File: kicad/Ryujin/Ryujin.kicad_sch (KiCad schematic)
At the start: 17 parts, among them J3 BAT, J4 SDI12, Q1 IRLML6244, U1 TXS0101DBV, U2 R-78E5.0-0.5, U3 W25Q32JVSS

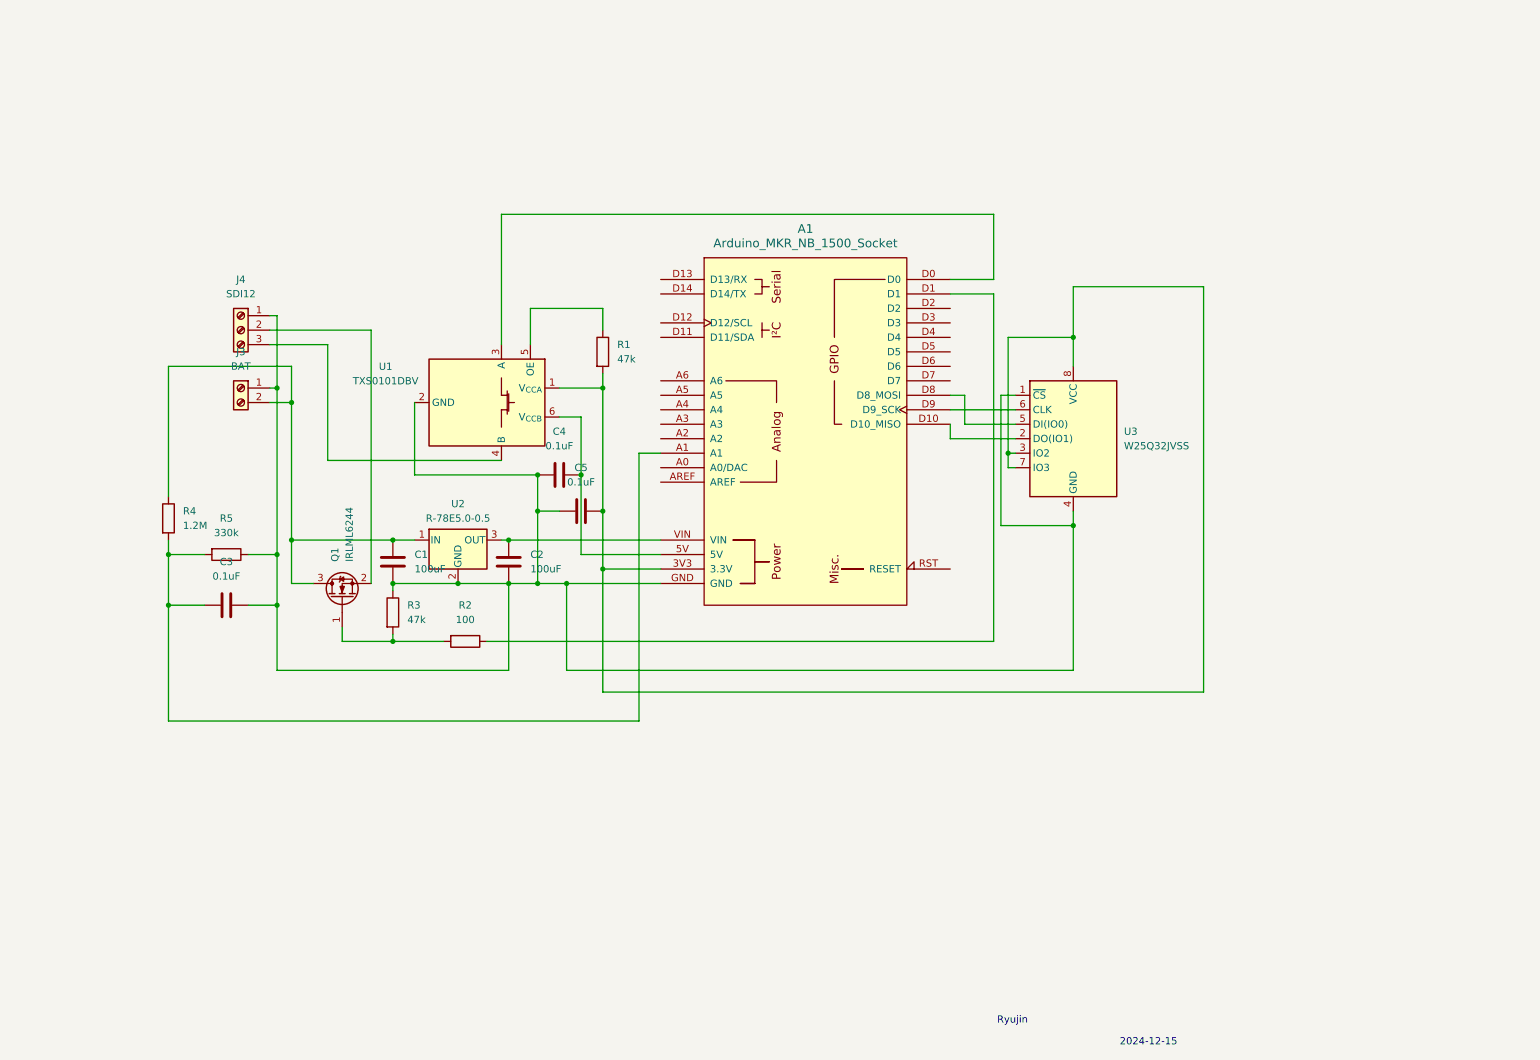
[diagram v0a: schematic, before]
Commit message: Ares
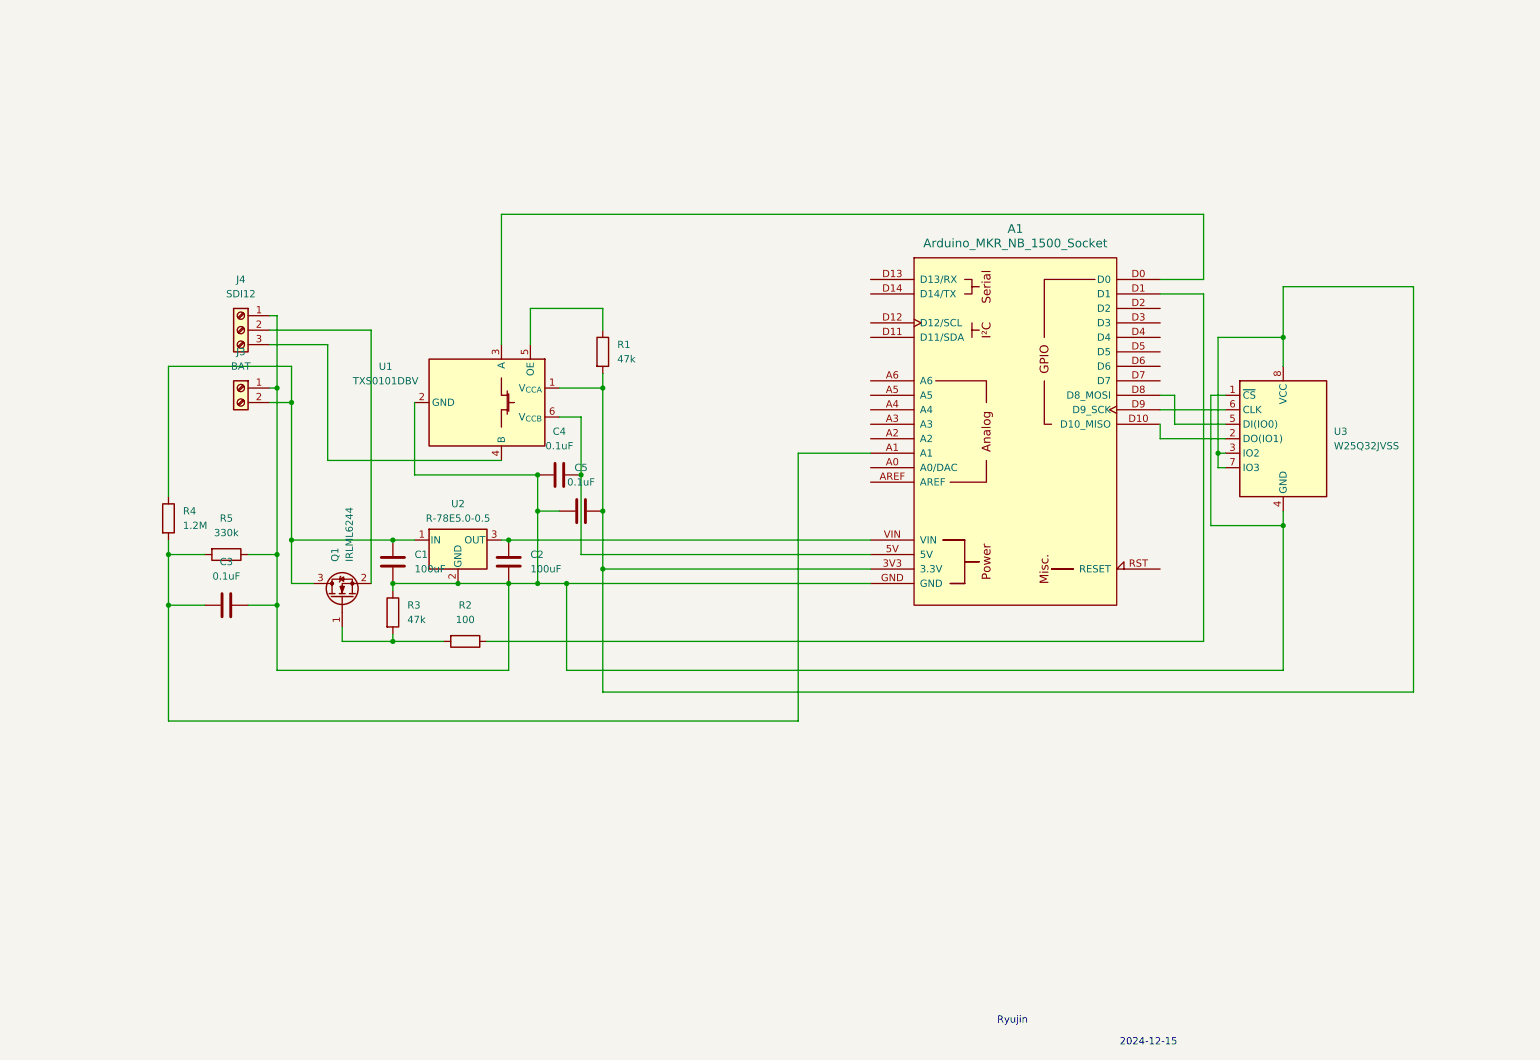
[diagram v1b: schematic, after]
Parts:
- C3: MPN 0.1uF 16V 0603 -> 0.1uF 0603 16V
- C4: MPN 0.1uF 6.3V 0603 -> 0.1uF 0603 6V
- C5: MPN 0.1uF 6.3V 0603 -> 0.1uF 0603 4V
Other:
- moved on the sheet: A1, U3

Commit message: Pride Comes Before a Brawl
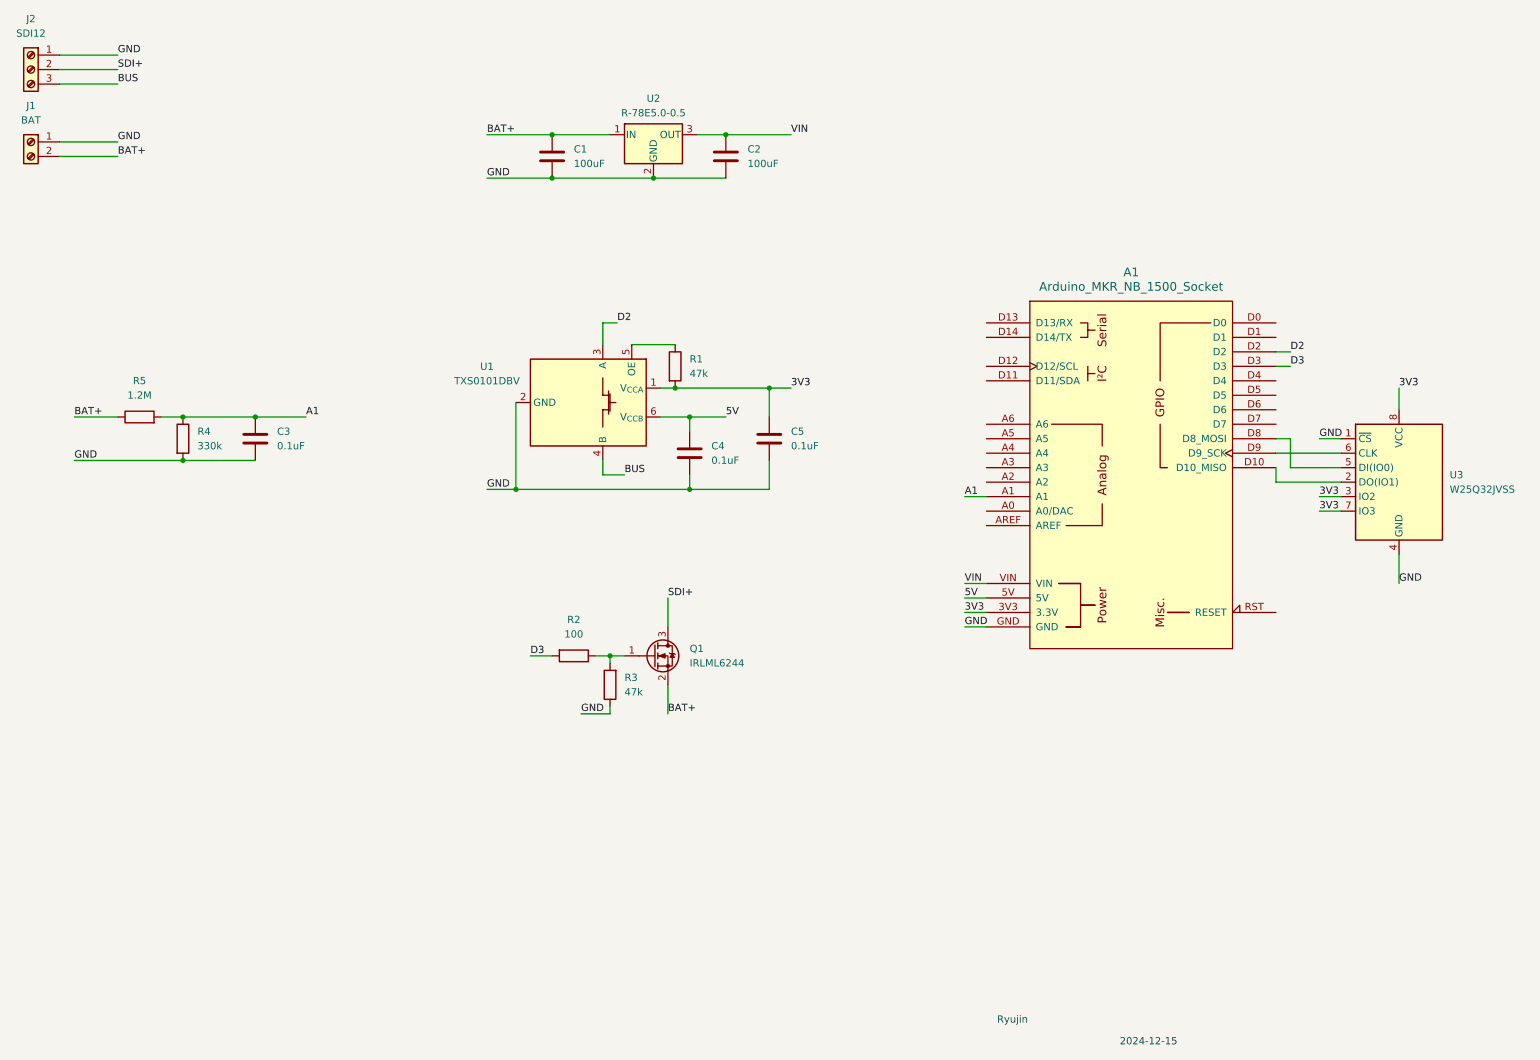
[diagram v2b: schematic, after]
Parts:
- A1: footprint PCM_arduino-library:Arduino_MKR_FOX_1200_Socket -> Custom:Arduino_MKR_NB_1500_Socket
- C3: MPN 0.1uF 0603 16V -> 0.1uF 16V 0603
- C4: MPN 0.1uF 0603 6V -> 0.1uF 6.3V 0603
- C5: MPN 0.1uF 0603 4V -> 0.1uF 6.3V 0603
- R4: value 1.2M -> 330k; MPN 1.2M 0603 -> 330k 0603
- R5: value 330k -> 1.2M; MPN 330k 0603 -> 1.2M 0603
- renumbered J3 to J1, J4 to J2
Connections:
- net 3V3: now reaches A1.3V3 (3.3V), C5.1, R1.2, U1.1 (V_{CCA}), U3.3 (IO2), U3.7 (IO3), U3.8 (VCC)
- net GND: now reaches A1.GND, C1.2, C2.2, C5.2, J1.1 (Pin_1), J2.1 (Pin_1), R3.1, U1.2 (GND), U2.2 (GND), U3.1 (~{CS}), U3.4 (GND)
- net GND: now also C3.2, C4.1, R4.2; no longer C3.1, C4.2, R5.1
- net at Q1.1 (G), R3.2: now also R2.1; no longer R2.2
- net BAT+: now reaches Q1.2 (S)
- net BAT+: now also C1.1, J1.2 (Pin_2), R5.1, U2.1 (IN); no longer J2.2 (Pin_2)
- net BUS: now reaches J2.3 (Pin_3), U1.4 (B)
- net at A1.D1: no longer R2.1
- net A1: now reaches A1.A1, R5.2
- net A1: now also C3.1, R4.1; no longer C3.2, R4.2
- net 5V: now reaches A1.5V, U1.6 (V_{CCB})
- net 5V: now also C4.2; no longer C4.1
- net VIN: now reaches A1.VIN, C2.1, U2.3 (OUT)
- net at A1.D0: no longer U1.3 (A)
- net D2: now reaches A1.D2
- net D2: now also U1.3 (A)
- net D3: now reaches A1.D3
- net D3: now also R2.2
- new net SDI+: J2.2 (Pin_2), Q1.3 (D)
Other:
- moved on the sheet: A1, C1, C2, J1, J2, U1, U2, U3
